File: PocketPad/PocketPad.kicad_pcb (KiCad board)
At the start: 2 copper layers, 71.6 x 62.7 mm, 35 parts, among them SW0 SW_Push, SW1 SW_Push, SW10 SW_Push, SW11 SW_Push, SW12 SW_Push, SW13 SW_Push, SW14 SW_Push, SW15 SW_Push, SW16 SW_Push, SW2 SW_Push, SW3 SW_Push, SW4 SW_Push, SW5 SW_Push, SW6 SW_Push, SW7 SW_Push, SW8 SW_Push, SW9 SW_Push

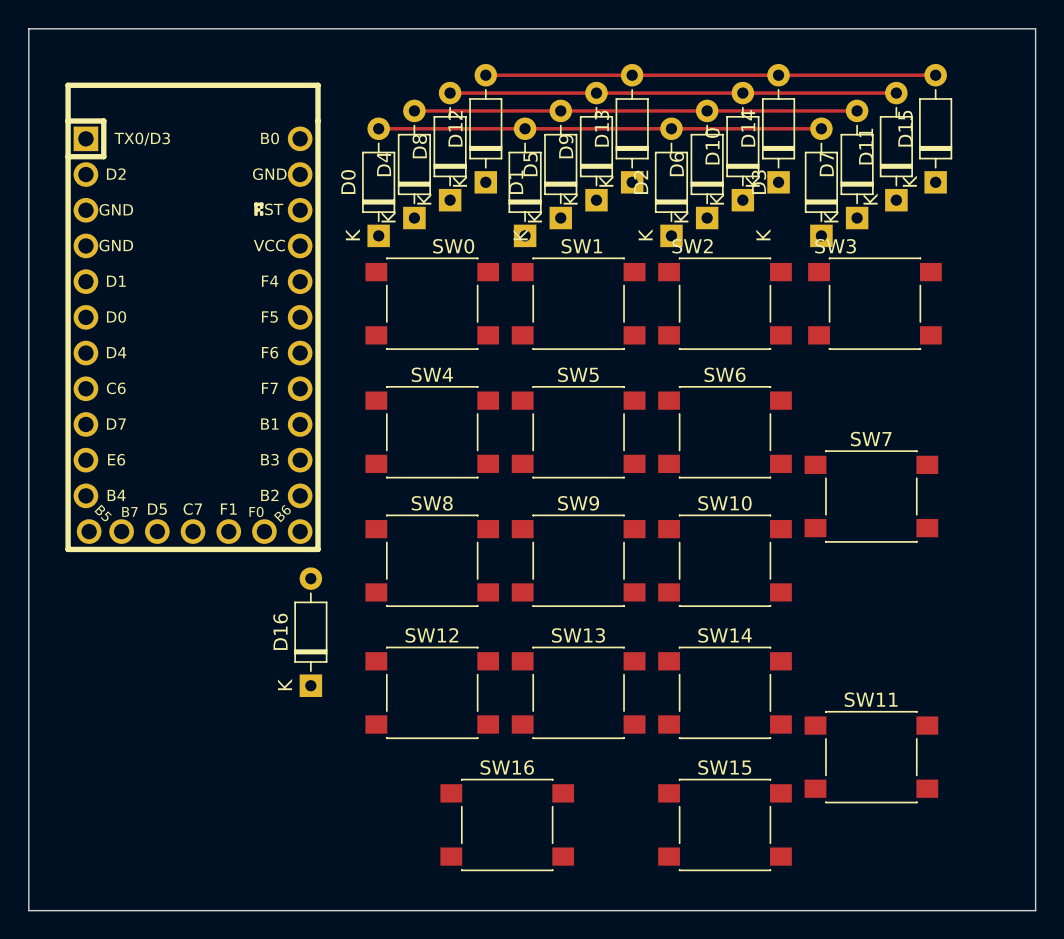
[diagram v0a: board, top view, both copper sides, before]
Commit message: V0.1 Complete
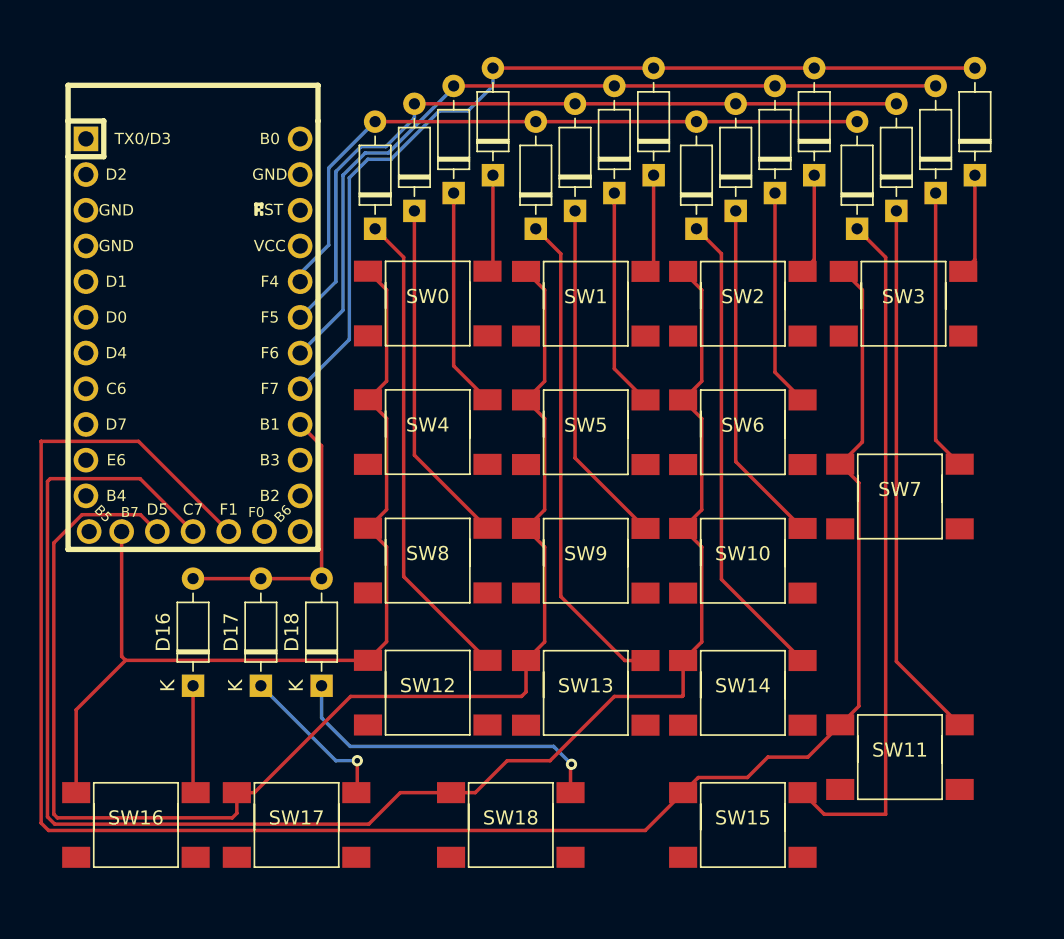
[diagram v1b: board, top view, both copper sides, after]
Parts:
- added D17: DIODE, Diode_THT:D_DO-35_SOD27_P7.62mm_Horizontal, F.Cu at (42.2, 82.5)
- added D18: DIODE, Diode_THT:D_DO-35_SOD27_P7.62mm_Horizontal, F.Cu at (46.5, 82.5)
- added SW17: SW_Push, Keebio:Switch_6x6x8.5, F.Cu at (44.7, 92.5)
- added SW18: SW_Push, Keebio:Switch_6x6x8.5, F.Cu at (59.9, 92.5)
- SW0, SW1, SW10, SW11, SW12, SW13, SW14, SW15, SW16, SW2, SW3, SW4, SW5, SW6, SW7, SW8, SW9: footprint Button_Switch_SMD:SW_SPST_PTS645 -> Keebio:Switch_6x6x8.5
- moved SW16 26.4 mm to (33.3, 92.5)
- moved D3 11.7 mm to (93.0, 46.2)
- moved D2 11.0 mm to (81.5, 46.2)
- moved D1 10.1 mm to (70.1, 46.2)
- moved D0 9.20 mm to (58.7, 46.2)
- moved D12 8.54 mm to (50.3, 50.0)
- moved D16 8.38 mm to (37.3, 82.5)
- moved D13 7.61 mm to (61.7, 50.0)
- moved D14 6.71 mm to (73.2, 50.0)
- moved D15 6.49 mm to (84.6, 50.0)
- moved D7 5.86 mm to (90.2, 47.5)
- moved D6 5.14 mm to (78.7, 47.5)
- moved D5 4.20 mm to (67.3, 47.5)
- moved D4 3.31 mm to (55.9, 47.5)
- moved D8 2.65 mm to (53.1, 48.8)
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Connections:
- D16 pad 2: unconnected-(D16-Pad2) -> ROW4
- MCU1 pad 16: unconnected-(MCU1-Pad16) -> ROW4
- MCU1 pad 17: unconnected-(MCU1-Pad17) -> ROW0
- MCU1 pad 18: unconnected-(MCU1-Pad18) -> ROW1
- MCU1 pad 19: unconnected-(MCU1-Pad19) -> ROW2
- MCU1 pad 20: unconnected-(MCU1-Pad20) -> ROW3
- MCU1 pad 25: unconnected-(MCU1-Pad25) -> COL0
- MCU1 pad 26: unconnected-(MCU1-Pad26) -> COL1
- MCU1 pad 27: unconnected-(MCU1-Pad27) -> COL2
- MCU1 pad 28: unconnected-(MCU1-Pad28) -> COL3
- SW0 pad 1: Net-(SW0-Pad1) -> COL0
- SW1 pad 1: Net-(SW1-Pad1) -> COL1
- SW10 pad 1: Net-(SW10-Pad1) -> COL2
- SW11 pad 1: Net-(SW11-Pad1) -> COL3
- SW12 pad 1: Net-(SW0-Pad1) -> COL0
- SW13 pad 1: Net-(SW1-Pad1) -> COL1
- SW14 pad 1: Net-(SW10-Pad1) -> COL2
- SW15 pad 1: Net-(SW11-Pad1) -> COL3
- SW16 pad 1: Net-(SW0-Pad1) -> COL0
- SW2 pad 1: Net-(SW10-Pad1) -> COL2
- SW3 pad 1: Net-(SW11-Pad1) -> COL3
- SW4 pad 1: Net-(SW0-Pad1) -> COL0
- SW5 pad 1: Net-(SW1-Pad1) -> COL1
- SW6 pad 1: Net-(SW10-Pad1) -> COL2
- SW7 pad 1: Net-(SW11-Pad1) -> COL3
- SW8 pad 1: Net-(SW0-Pad1) -> COL0
- SW9 pad 1: Net-(SW1-Pad1) -> COL1
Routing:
- net COL3: track 0.00 -> 137.9 mm
- net COL2: track 0.00 -> 118.6 mm
- net COL1: track 0.00 -> 99.5 mm
- net COL0: track 0.00 -> 68.4 mm
- net Net-(D15-Pad1): track 0.00 -> 49.0 mm
- net Net-(D11-Pad1): track 0.00 -> 38.4 mm
- net Net-(D13-Pad1): track 0.00 -> 34.8 mm
- net Net-(D12-Pad1): track 0.00 -> 34.0 mm
- net Net-(D14-Pad1): track 0.00 -> 33.8 mm
- net ROW0: track 31.5 -> 64.7 mm
- net ROW1: track 31.5 -> 58.8 mm
- net Net-(D8-Pad1): track 0.00 -> 24.7 mm
- net Net-(D9-Pad1): track 0.00 -> 24.7 mm
- net Net-(D10-Pad1): track 0.00 -> 24.6 mm
- net Net-(D18-Pad1): track 0.00 -> 23.5 mm, vias 0 -> 1
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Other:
- board outline removed
